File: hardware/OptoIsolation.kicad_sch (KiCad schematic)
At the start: 8 parts, among them U10 TLP293-4, U9 TLP293-4

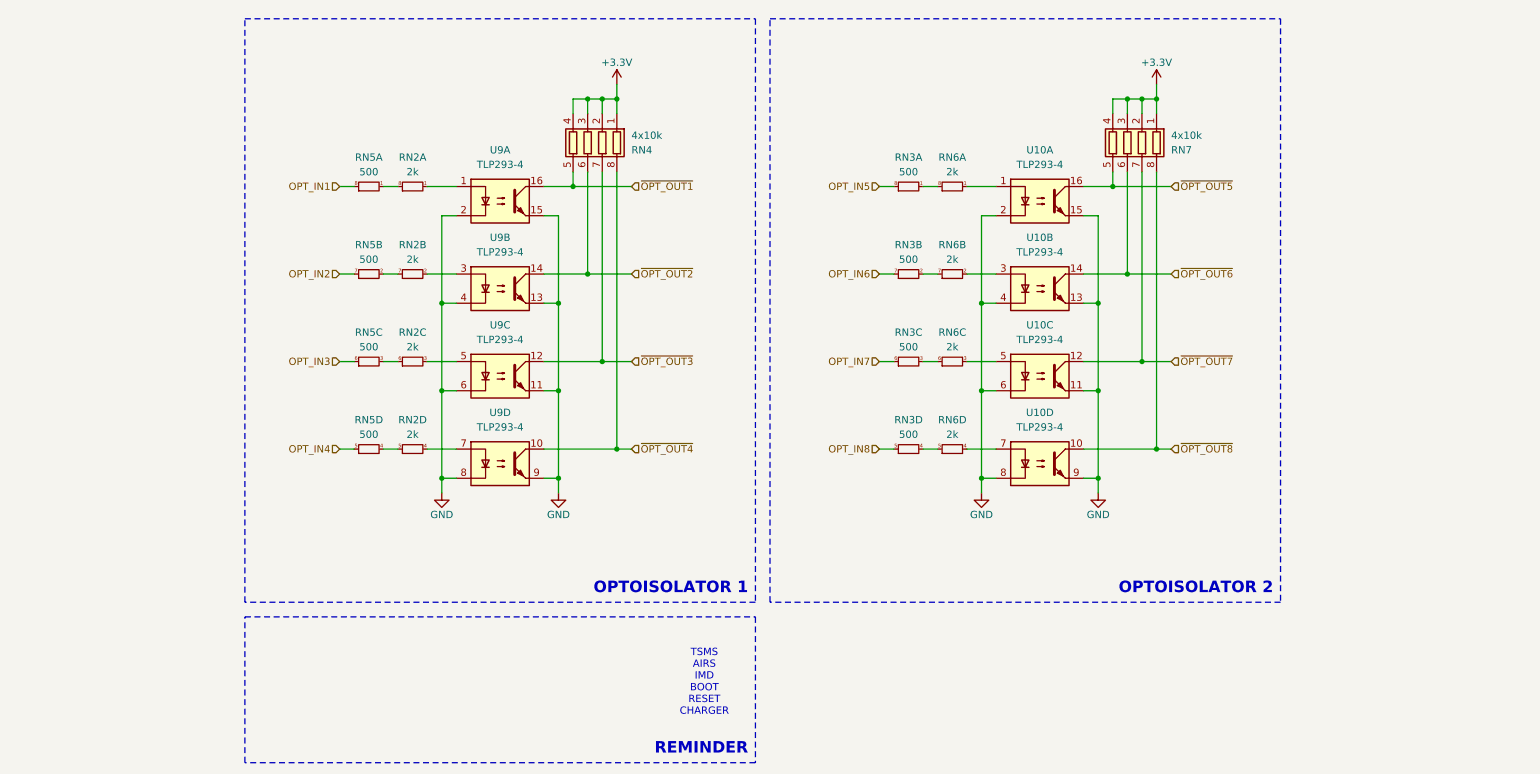
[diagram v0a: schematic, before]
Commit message: sync
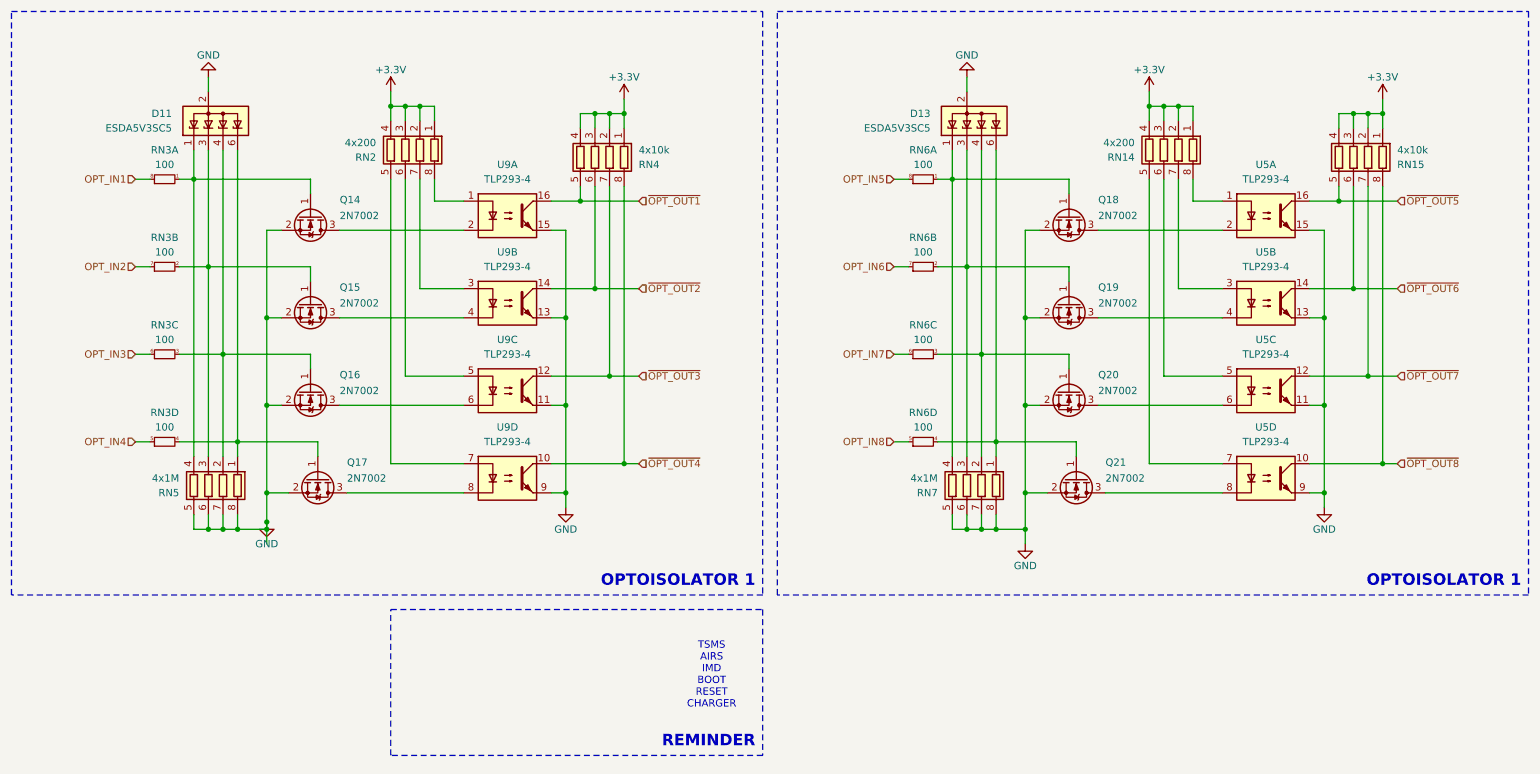
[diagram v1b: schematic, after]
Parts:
- removed RN2: 2k, Resistor_SMD:R_Array_Convex_4x0603, symbol Device:R_Pack04_Split
- removed RN5: 500, Resistor_SMD:R_Array_Convex_4x0603, symbol Device:R_Pack04_Split
- removed U10: TLP293-4, Package_SO:SOIC-16_4.55x10.3mm_P1.27mm, symbol Isolator:TLP293-4
- added D11, D13: ESDA5V3SC5, Package_TO_SOT_SMD:SOT-23-6, symbol Power_Protection:ESDA5V3SC5
- added Q14, Q15, Q16, Q17, Q18, Q19, Q20, Q21: 2N7002, Package_TO_SOT_SMD:SOT-23, symbol Transistor_FET:2N7002
- added RN14, RN2: 4x200, Resistor_SMD:R_Array_Convex_4x0603, symbol Device:R_Pack04
- added RN15: 4x10k, Resistor_SMD:R_Array_Convex_4x0603, symbol Device:R_Pack04
- added RN5: 4x1M, Resistor_SMD:R_Array_Convex_4x0603, symbol Device:R_Pack04
- added U5: TLP293-4, Package_SO:SOIC-16_4.55x10.3mm_P1.27mm, symbol Isolator:TLP293-4
- RN3: value 500 -> 100
- RN6: value 2k -> 100
- RN7: value 4x10k -> 4x1M
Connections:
- net +3.3V: now also RN14.1 (R1.1), RN14.2 (R2.1), RN14.3 (R3.1), RN14.4 (R4.1), RN15.1 (R1.1), RN15.2 (R2.1), RN15.3 (R3.1), RN15.4 (R4.1), RN2.1 (R1.1), RN2.2 (R2.1), RN2.3 (R3.1), RN2.4 (R4.1); no longer RN7.1 (R1.1), RN7.2 (R2.1), RN7.3 (R3.1), RN7.4 (R4.1)
- net GND: now also RN7.5 (R4.2), RN7.6 (R3.2), RN7.7 (R2.2), RN7.8 (R1.2), D11.2 (K), D11.5 (NC), D13.2 (K), D13.5 (NC), Q14.2 (S), Q15.2 (S), Q16.2 (S), Q17.2 (S), Q18.2 (S), Q19.2 (S), Q20.2 (S), Q21.2 (S), RN5.5 (R4.2), RN5.6 (R3.2), RN5.7 (R2.2), RN5.8 (R1.2), U5.11, U5.13, U5.15, U5.9; no longer U9.2, U9.4, U9.6, U9.8
- net OPT_IN1: now also RN3.8 (R1.2)
- net OPT_IN2: now also RN3.7 (R2.2)
- net OPT_IN3: now also RN3.6 (R3.2)
- net OPT_IN4: now also RN3.5 (R4.2)
- net OPT_IN5: now also RN6.8 (R1.2); no longer RN3.8 (R1.2)
- net OPT_IN6: now also RN6.7 (R2.2); no longer RN3.7 (R2.2)
- net OPT_IN7: now also RN6.6 (R3.2); no longer RN3.6 (R3.2)
- net OPT_IN8: now also RN6.5 (R4.2); no longer RN3.5 (R4.2)
- net ~{OPT_OUT5}: now also RN15.5 (R4.2), U5.16; no longer RN7.5 (R4.2)
- net ~{OPT_OUT6}: now also RN15.6 (R3.2), U5.14; no longer RN7.6 (R3.2)
- net ~{OPT_OUT7}: now also RN15.7 (R2.2), U5.12; no longer RN7.7 (R2.2)
- net ~{OPT_OUT8}: now also RN15.8 (R1.2), U5.10; no longer RN7.8 (R1.2)
- net at U9.1: now also RN2.8 (R1.2)
- net at RN6.1 (R1.1): now also RN7.4 (R4.1), D13.1 (A), Q18.1 (G)
- net at RN6.3 (R3.1): now also RN7.2 (R2.1), D13.4 (A), Q20.1 (G)
- net at U9.5: now also RN2.6 (R3.2)
- net at RN6.4 (R4.1): now also RN7.1 (R1.1), D13.6 (A), Q21.1 (G)
- net at RN3.4 (R4.1): now also D11.6 (A), Q17.1 (G), RN5.1 (R1.1); no longer RN6.5 (R4.2)
- net at RN6.2 (R2.1): now also RN7.3 (R3.1), D13.3 (A), Q19.1 (G)
- net at RN3.2 (R2.1): now also D11.3 (A), Q15.1 (G), RN5.3 (R3.1); no longer RN6.7 (R2.2)
- net at RN3.1 (R1.1): now also D11.1 (A), Q14.1 (G), RN5.4 (R4.1); no longer RN6.8 (R1.2)
- net at U9.3: now also RN2.7 (R2.2)
- net at U9.7: now also RN2.5 (R4.2)
- net at RN3.3 (R3.1): now also D11.4 (A), Q16.1 (G), RN5.2 (R2.1); no longer RN6.6 (R3.2)
- new net: Q19.3 (D), U5.4
- new net: Q16.3 (D), U9.6
- new net: Q20.3 (D), U5.6
- new net: Q15.3 (D), U9.4
- new net: RN14.5 (R4.2), U5.7
- new net: Q21.3 (D), U5.8
- new net: RN14.7 (R2.2), U5.3
- new net: Q14.3 (D), U9.2
- new net: RN14.8 (R1.2), U5.1
- new net: Q18.3 (D), U5.2
- new net: RN14.6 (R3.2), U5.5
- new net: Q17.3 (D), U9.8
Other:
- note removed: "OPTOISOLATOR 2"
- moved on the sheet: RN4, U9A, U9B, U9C, U9D

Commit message: schematic done
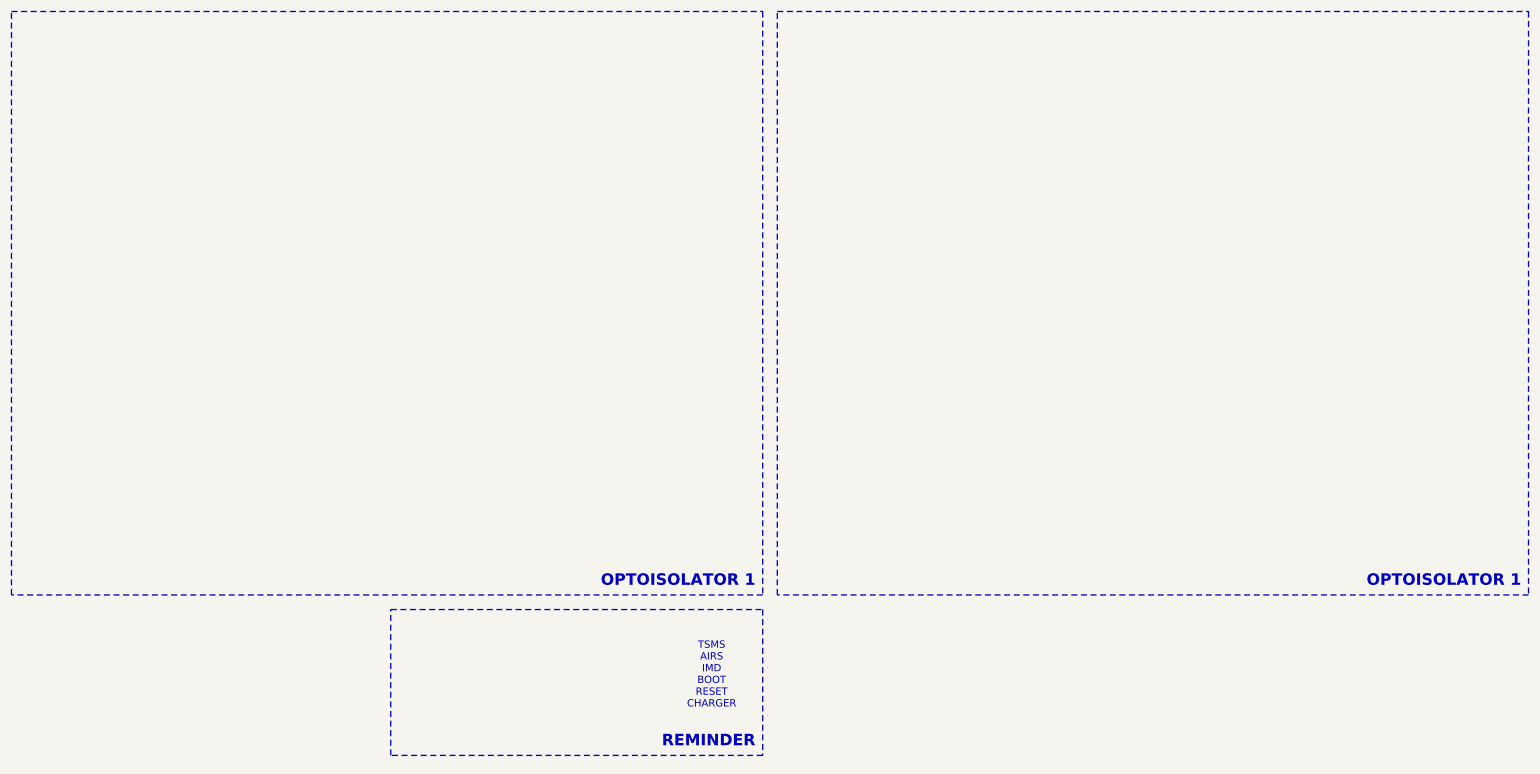
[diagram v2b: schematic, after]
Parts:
- removed D11, D13: ESDA5V3SC5, Package_TO_SOT_SMD:SOT-23-6, symbol Power_Protection:ESDA5V3SC5
- removed Q14, Q15, Q16, Q17, Q18, Q19, Q20, Q21: 2N7002, Package_TO_SOT_SMD:SOT-23, symbol Transistor_FET:2N7002
- removed RN14, RN2: 4x200, Resistor_SMD:R_Array_Convex_4x0603, symbol Device:R_Pack04
- removed RN15, RN4: 4x10k, Resistor_SMD:R_Array_Convex_4x0603, symbol Device:R_Pack04
- removed RN3, RN6: 100, Resistor_SMD:R_Array_Convex_4x0603, symbol Device:R_Pack04_Split
- removed RN5, RN7: 4x1M, Resistor_SMD:R_Array_Convex_4x0603, symbol Device:R_Pack04
- removed U5, U9: TLP293-4, Package_SO:SOIC-16_4.55x10.3mm_P1.27mm, symbol Isolator:TLP293-4
